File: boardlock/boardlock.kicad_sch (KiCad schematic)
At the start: 7 parts, among them U1 ESP32-S3-WROOM-1

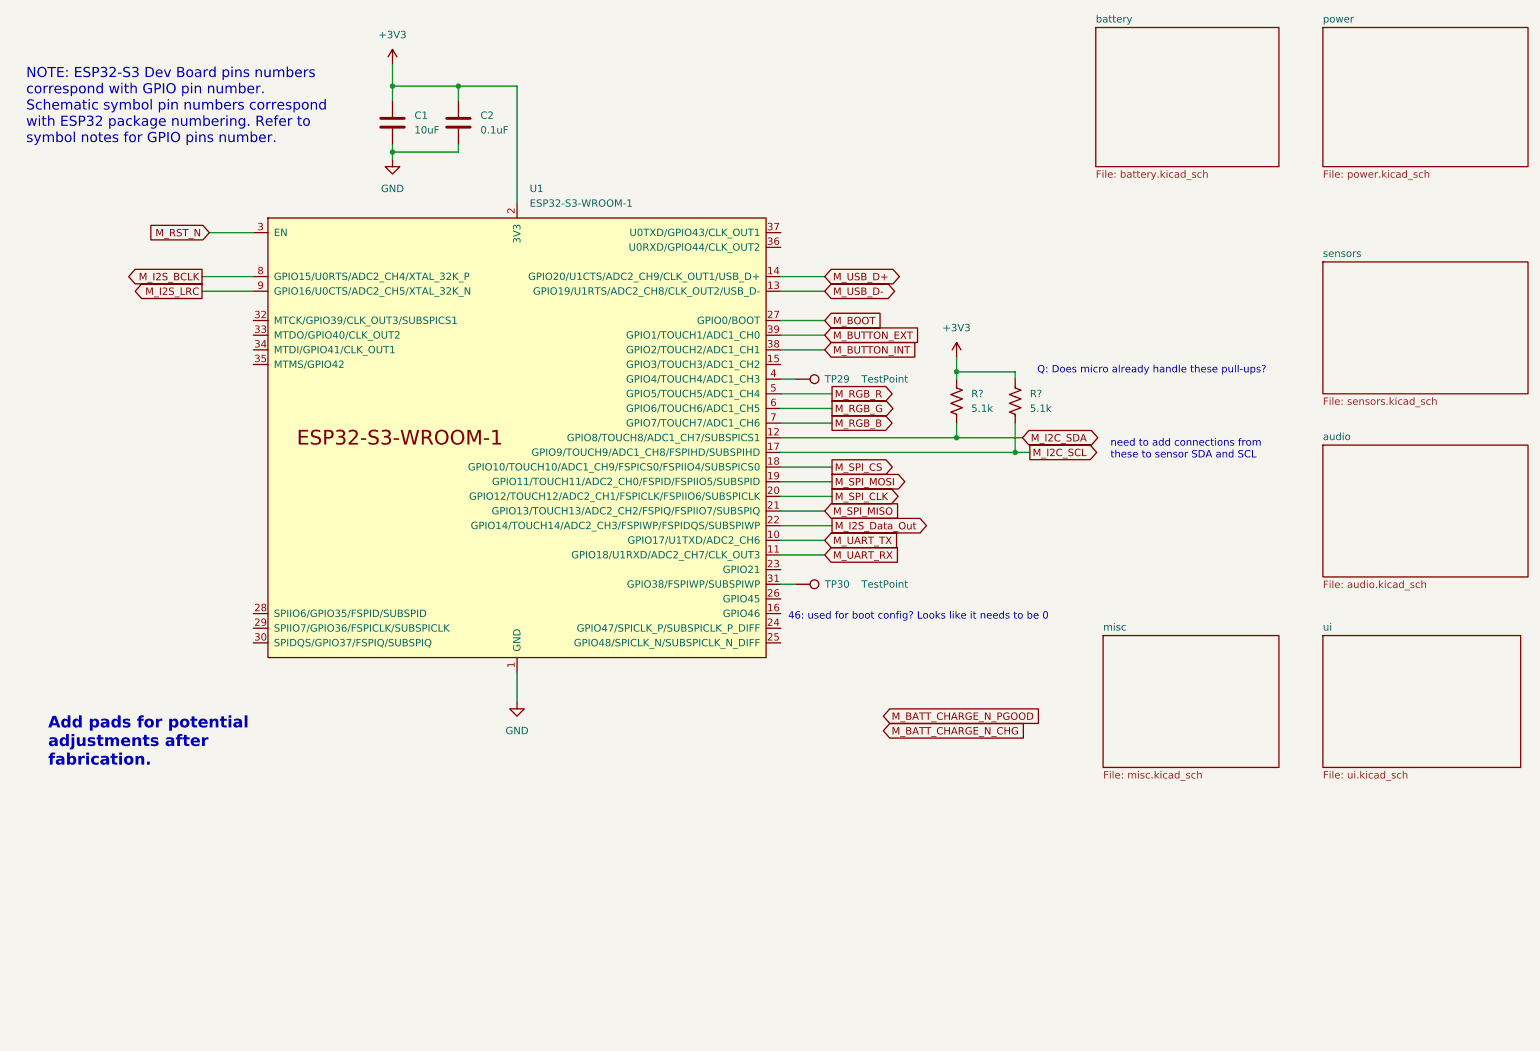
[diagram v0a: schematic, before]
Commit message: lab updates
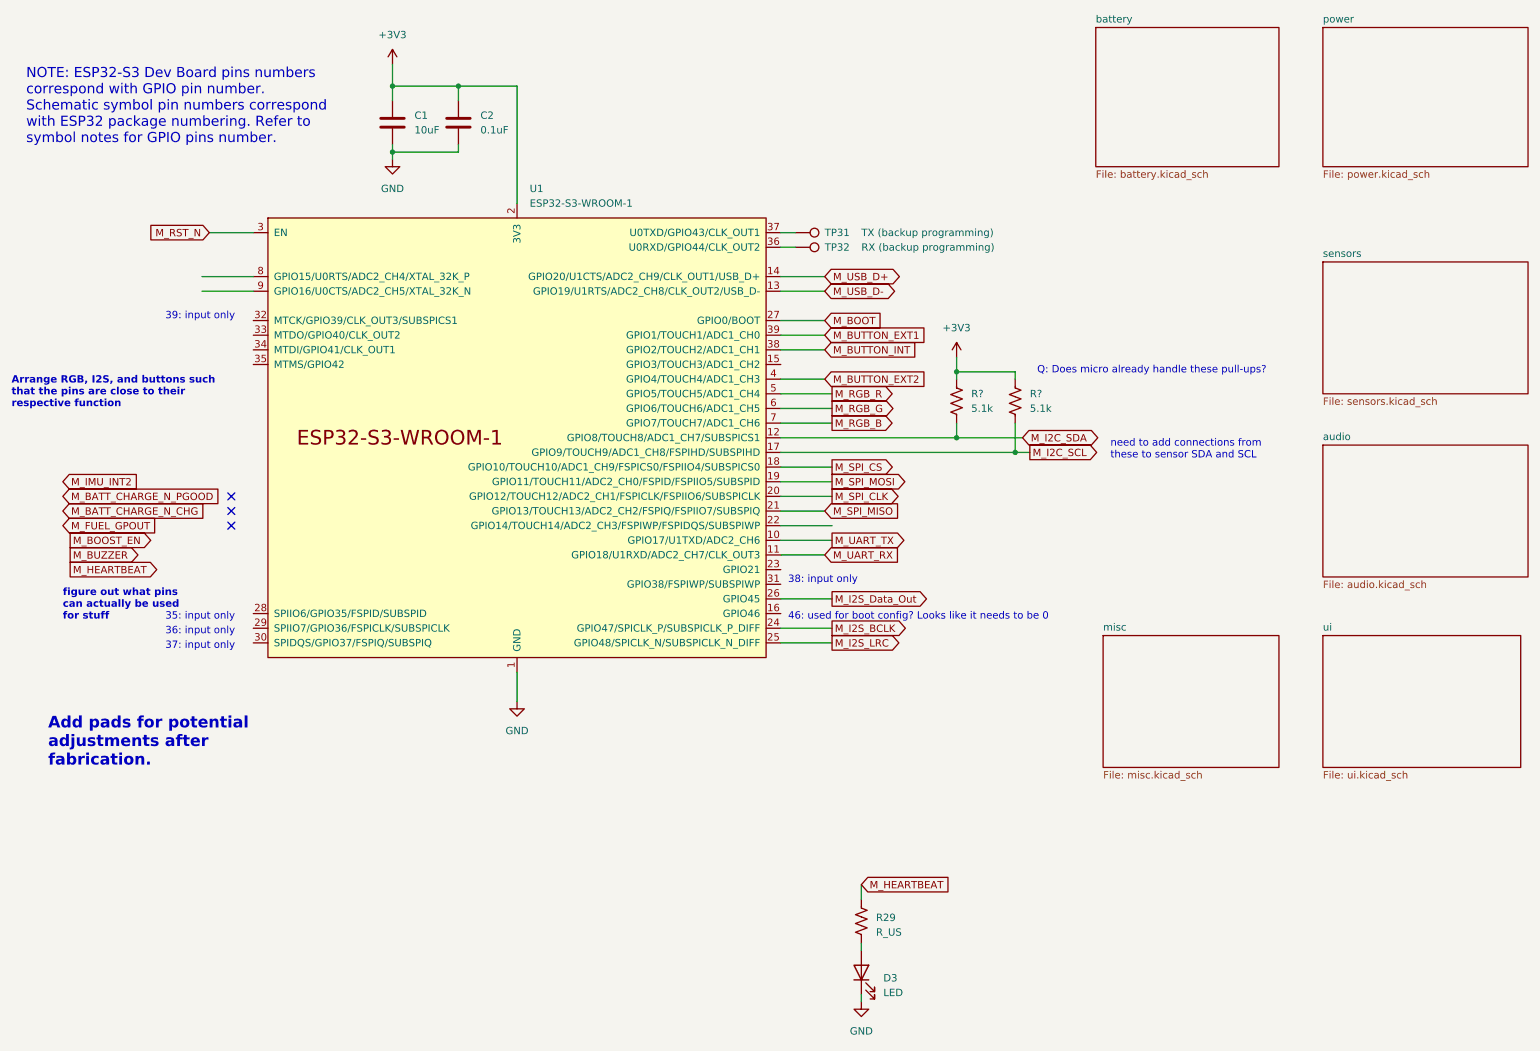
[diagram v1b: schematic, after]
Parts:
- removed TP29, TP30: TestPoint, symbol Connector:TestPoint
- added D3: LED, symbol Device:LED
- added R29: R_US, symbol Device:R_US
- added TP31: TX (backup programming), symbol Connector:TestPoint
- added TP32: RX (backup programming), symbol Connector:TestPoint
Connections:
- net GND: now also D3.1 (K)
- net M_I2S_BCLK: now also U1.24 (GPIO47/SPICLK_P/SUBSPICLK_P_DIFF); no longer U1.8 (GPIO15/U0RTS/ADC2_CH4/XTAL_32K_P)
- net M_I2S_Data_Out: now also U1.26 (GPIO45); no longer U1.22 (GPIO14/TOUCH14/ADC2_CH3/FSPIWP/FSPIDQS/SUBSPIWP)
- net M_I2S_LRC: now also U1.25 (GPIO48/SPICLK_N/SUBSPICLK_N_DIFF); no longer U1.9 (GPIO16/U0CTS/ADC2_CH5/XTAL_32K_N)
- net M_BUTTON_EXT2: now reaches U1.4 (GPIO4/TOUCH4/ADC1_CH3)
- net at U1.36 (U0RXD/GPIO44/CLK_OUT2): now also TP32.1
- net at U1.37 (U0TXD/GPIO43/CLK_OUT1): now also TP31.1
- net M_BUTTON_EXT renamed M_BUTTON_EXT1
- new net: D3.2 (A), R29.2
- new net M_HEARTBEAT: R29.1
- no-connect marks 0 -> 3
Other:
- note added: "35: input only"
- note added: "36: input only"
- note added: "37: input only"
- note added: "38: input only"
- note added: "39: input only"
- note added: "Arrange RGB, I2S, and buttons such that the pins are close to their respective function"
- note added: "figure out what pins can actually be used for stuff"
